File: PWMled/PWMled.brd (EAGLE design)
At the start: 9.1 x 10.9 mm, 6 parts, among them T1 BCX19

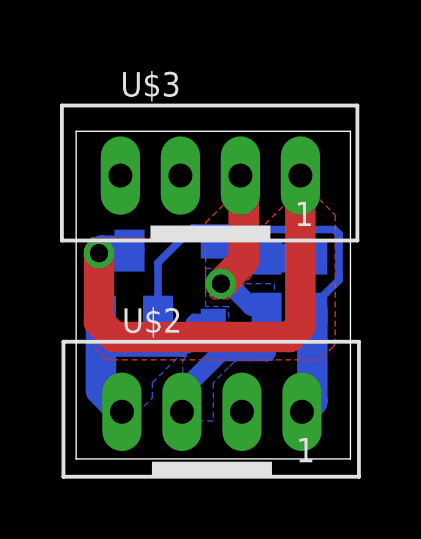
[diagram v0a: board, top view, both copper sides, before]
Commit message: some cleanup
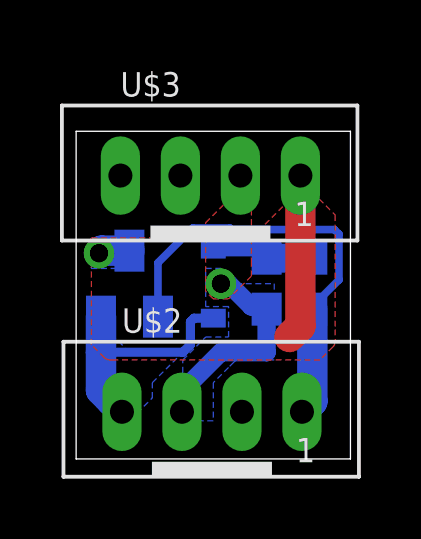
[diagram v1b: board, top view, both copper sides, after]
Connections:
- net N$1 renamed 3.3V
- net N$2 renamed LED-
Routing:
- net LED-: track 15.6 -> 6.79 mm
- net 12V: track 11.4 -> 7.47 mm
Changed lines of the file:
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@@
 <?xml version="1.0" encoding="utf-8"?>
 <!DOCTYPE eagle SYSTEM "eagle.dtd">
-<eagle version="6.4">
+<eagle version="9.0.0">
 <drawing>
 <settings>
 <setting alwaysvectorfont="no"/>
+<setting keepoldvectorfont="yes"/>
 <setting verticaltext="up"/>
 </settings>
@@
 <layers>
 <layer number="1" name="Top" color="4" fill="1" visible="yes" active="yes"/>
-<layer number="16" name="Bottom" color="1" fill="1" visible="no" active="yes"/>
+<layer number="16" name="Bottom" color="1" fill="1" visible="yes" active="yes"/>
 <layer number="17" name="Pads" color="2" fill="1" visible="yes" active="yes"/>
 <layer number="18" name="Vias" color="2" fill="1" visible="yes" active="yes"/>
@@
 <param name="dpMaxLengthDifference" value="10mm"/>
 <param name="dpGapFactor" value="2.5"/>
-<param name="checkGrid" value="0"/>
 <param name="checkAngle" value="0"/>
 <param name="checkFont" value="1"/>
 <param name="checkRestrict" value="1"/>
+<param name="checkStop" value="0"/>
+<param name="checkValues" value="0"/>
 <param name="useDiameter" value="13"/>
 <param name="maxErrors" value="50"/>
@@
 <pass name="Default">
 <param name="RoutingGrid" value="50mil"/>
+<param name="AutoGrid" value="1"/>
+<param name="Efforts" value="0"/>
+<param name="TopRouterVariant" value="1"/>
 <param name="tpViaShape" value="round"/>
 <param name="PrefDir.1" value="|"/>
@@
 </elements>
 <signals>
-<signal name="N$1">
+<signal name="3.3V">
 <contactref element="R1" pad="1"/>
 <contactref element="R2" pad="1"/>
@@
 </signal>
 <signal name="PWM">
-<contactref element="R2" pad="2"/>
 <contactref element="T1" pad="1"/>
 <contactref element="U$2" pad="P1"/>
@@
 <wire x1="8.6106" y1="7.6454" x2="8.763" y2="7.493" width="0.254" layer="16"/>
 <wire x1="8.128" y1="5.334" x2="8.128" y2="5.246" width="0.254" layer="16"/>
-<wire x1="8.128" y1="5.246" x2="7.874" y2="4.992" width="0.254" layer="16"/>
-<wire x1="7.874" y1="4.992" x2="7.874" y2="1.9189" width="1.016" layer="16"/>
-<wire x1="7.874" y1="1.9189" x2="7.5266" y2="1.5715" width="1.016" layer="16"/>
+<contactref element="R2" pad="2"/>
+<wire x1="7.5266" y1="1.5715" x2="7.874" y2="1.9189" width="1.016" layer="16"/>
+<wire x1="7.874" y1="1.9189" x2="7.874" y2="4.992" width="1.016" layer="16"/>
+<wire x1="7.874" y1="4.992" x2="7.874" y2="5.08" width="0.254" layer="16"/>
+<wire x1="7.874" y1="5.08" x2="8.128" y2="5.334" width="0.254" layer="16"/>
 </signal>
 <signal name="12V">
@@
 <contactref element="U$2" pad="P3"/>
 <wire x1="5.4758" y1="9.4455" x2="5.588" y2="9.4455" width="1.016" layer="1"/>
-<wire x1="5.588" y1="9.4455" x2="5.588" y2="6.604" width="1.016" layer="1"/>
-<wire x1="5.588" y1="6.604" x2="4.826" y2="5.842" width="1.016" layer="1"/>
 <via x="4.826" y="5.842" extent="1-16" drill="0.6"/>
 <wire x1="4.826" y1="5.842" x2="5.08" y2="5.842" width="0.6096" layer="16"/>
@@
 </polygon>
 </signal>
-<signal name="N$2">
+<signal name="LED-">
 <contactref element="T1" pad="3"/>
 <contactref element="U$3" pad="P1"/>
@@
 <wire x1="7.4758" y1="9.4455" x2="7.4758" y2="4.4278" width="1.016" layer="1"/>
 <wire x1="7.4758" y1="4.4278" x2="7.112" y2="4.064" width="1.016" layer="1"/>
-<wire x1="7.112" y1="4.064" x2="1.27" y2="4.064" width="1.016" layer="1"/>
-<wire x1="1.27" y1="4.064" x2="0.762" y2="4.572" width="1.016" layer="1"/>
-<wire x1="0.762" y1="4.572" x2="0.762" y2="6.858" width="1.016" layer="1"/>
 <via x="0.762" y="6.858" extent="1-16" drill="0.6"/>
 <polygon width="0.508" layer="16" isolate="0.3048" thermals="no" rank="3">

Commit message: more cleanup
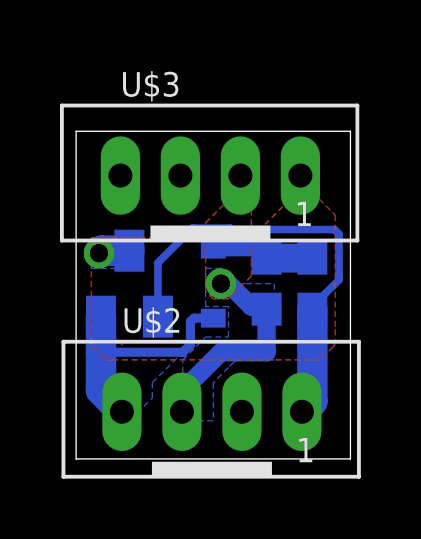
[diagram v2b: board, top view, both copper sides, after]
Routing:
- net LED-: track 6.79 -> 1.25 mm
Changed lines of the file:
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@@
 <via x="0.762" y="6.858" extent="1-16" drill="0.6"/>
 <wire x1="7.62" y1="9.3013" x2="7.4758" y2="9.4455" width="1.016" layer="1"/>
-<wire x1="7.4758" y1="9.4455" x2="7.4758" y2="4.4278" width="1.016" layer="1"/>
-<wire x1="7.4758" y1="4.4278" x2="7.112" y2="4.064" width="1.016" layer="1"/>
 <via x="0.762" y="6.858" extent="1-16" drill="0.6"/>
 <polygon width="0.508" layer="16" isolate="0.3048" thermals="no" rank="3">
